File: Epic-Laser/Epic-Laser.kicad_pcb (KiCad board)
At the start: 2 copper layers, 10 parts, among them J1 ICSP-Header, U1 PIC24FJ64GA002-I_SP, X1 USB-B1HSB6

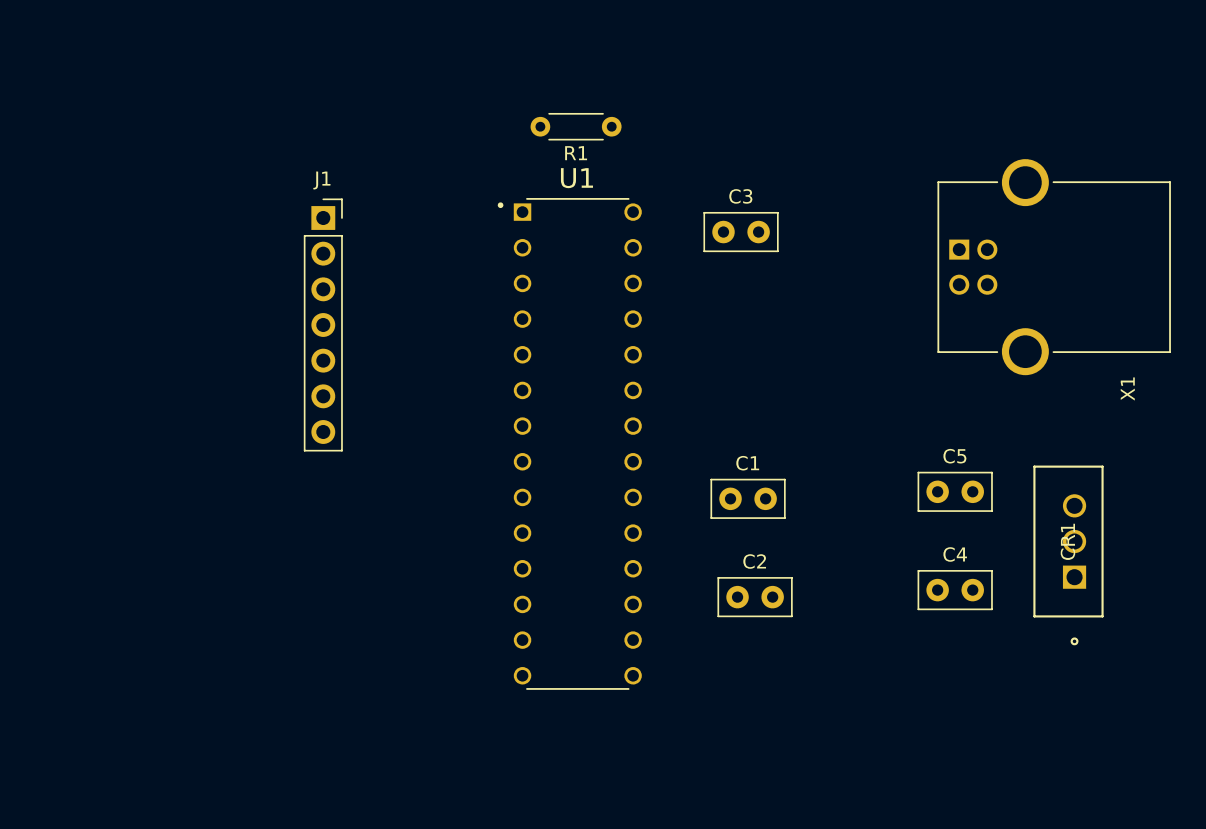
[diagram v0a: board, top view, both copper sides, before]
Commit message: Draft-Board-Layout
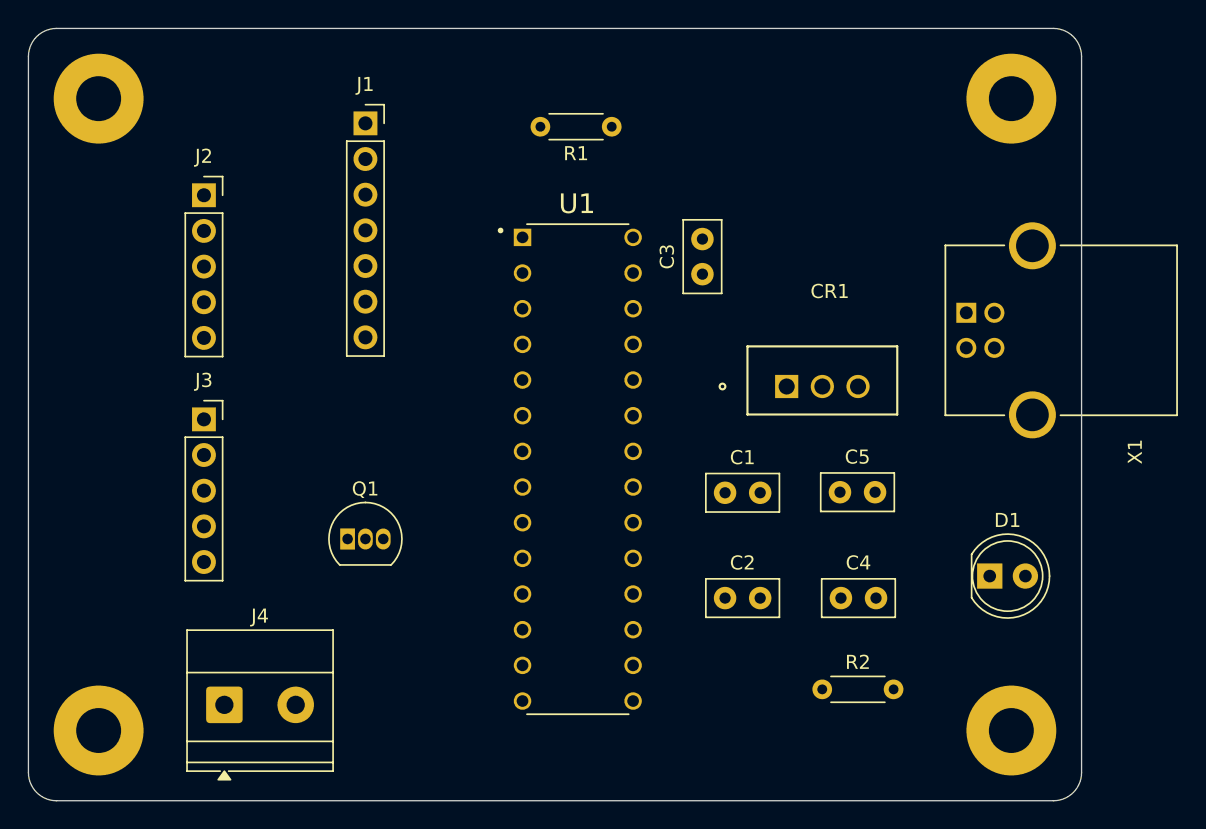
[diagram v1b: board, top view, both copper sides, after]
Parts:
- added D1: LED, LED_THT:LED_D5.0mm, F.Cu at (163.5, 94.0)
- added J2: X-Motor, Connector_PinSocket_2.54mm:PinSocket_1x05_P2.54mm_Vertical, F.Cu at (107.5, 66.9)
- added J3: Y-Motor, Connector_PinSocket_2.54mm:PinSocket_1x05_P2.54mm_Vertical, F.Cu at (107.5, 82.8)
- added J4: Laser_Control, TerminalBlock_Phoenix:TerminalBlock_Phoenix_MKDS-1,5-2-5.08_1x02_P5.08mm_Horizontal, F.Cu at (109.0, 103.2)
- added Q1: 2N7000, Package_TO_SOT_THT:TO-92_Inline, F.Cu at (117.7, 91.4)
- added R2: 1k, Resistor_THT:R_Axial_DIN0204_L3.6mm_D1.6mm_P5.08mm_Horizontal, F.Cu at (151.5, 102.1)
- added REF**: MountingHole_3.2mm_M3_Pad, MountingHole:MountingHole_3.2mm_M3_Pad, F.Cu at (165.0, 105.0)
- added REF**: MountingHole_3.2mm_M3_Pad, MountingHole:MountingHole_3.2mm_M3_Pad, F.Cu at (165.0, 60.0)
- added REF**: MountingHole_3.2mm_M3_Pad, MountingHole:MountingHole_3.2mm_M3_Pad, F.Cu at (100.0, 60.0)
- added REF**: MountingHole_3.2mm_M3_Pad, MountingHole:MountingHole_3.2mm_M3_Pad, F.Cu at (100.0, 105.0)
- moved CR1 24.6 mm to (149.0, 80.5), turned to 0 degrees
- moved J1 7.38 mm to (119.0, 61.8)
- moved C5 6.96 mm to (152.8, 88.0)
- moved C4 6.91 mm to (152.9, 95.6)
- moved X1 4.53 mm to (166.5, 76.5)
- moved C3 3.35 mm to (143.0, 72.5), turned to 90 degrees
- moved U1 1.80 mm to (134.1, 86.4)
- moved C2 0.89 mm to (144.6, 95.6)
- moved C1 0.58 mm to (144.6, 88.1)
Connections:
- U1 pad 14: unconnected-(U1-PGD3/EMUD3/RP5/ASDA1/CN27/PMD7/RB5-Pad14) -> /Laser_Drive
- U1 pad 15: unconnected-(U1-PGC3/EMUC3/RP6/ASCL1/CN24/PMD6/RB6-Pad15) -> /X_STEP
- U1 pad 16: unconnected-(U1-RP7/INT0/CN23/PMD5/RB7-Pad16) -> /Y_STEP
- U1 pad 17: unconnected-(U1-TCK/RP8/SCL1/CN22/PMD4/RB8-Pad17) -> /X_DIR
- U1 pad 18: unconnected-(U1-TDO/RP9/SDA1/CN21/PMD3/RB9-Pad18) -> /Y_DIR
- U1 pad 21: unconnected-(U1-PGD2/EMUD2/TDI/RP10/CN16/PMD2/RB10-Pad21) -> /X_EN
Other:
- board outline added: 75 x 55 mm
